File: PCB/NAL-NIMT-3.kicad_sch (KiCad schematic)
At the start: 27 parts

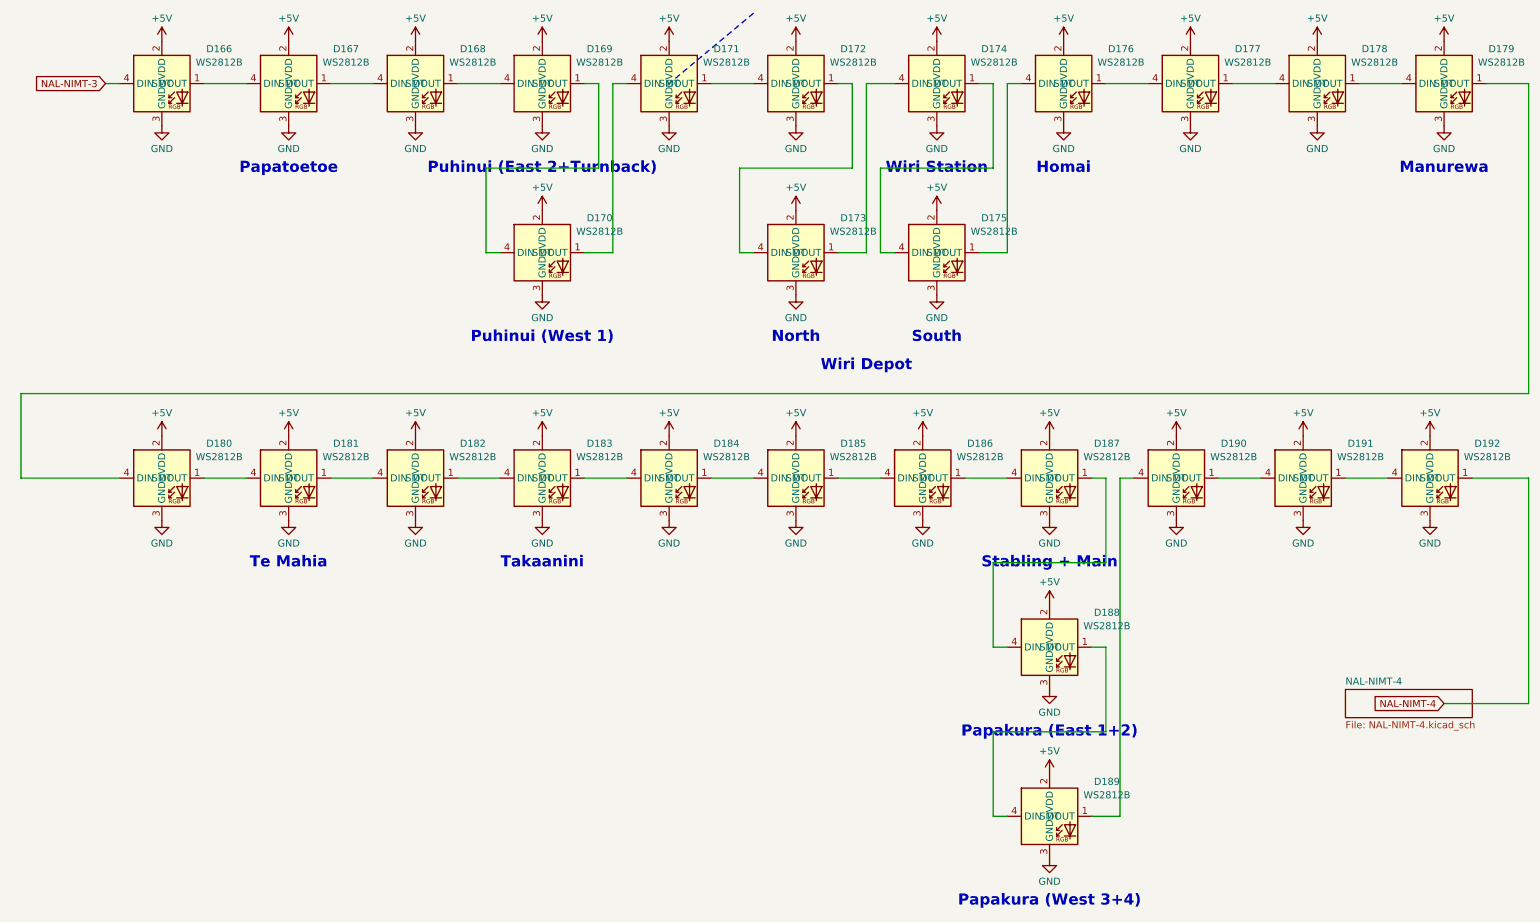
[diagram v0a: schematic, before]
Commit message: V1.1.0 PCB
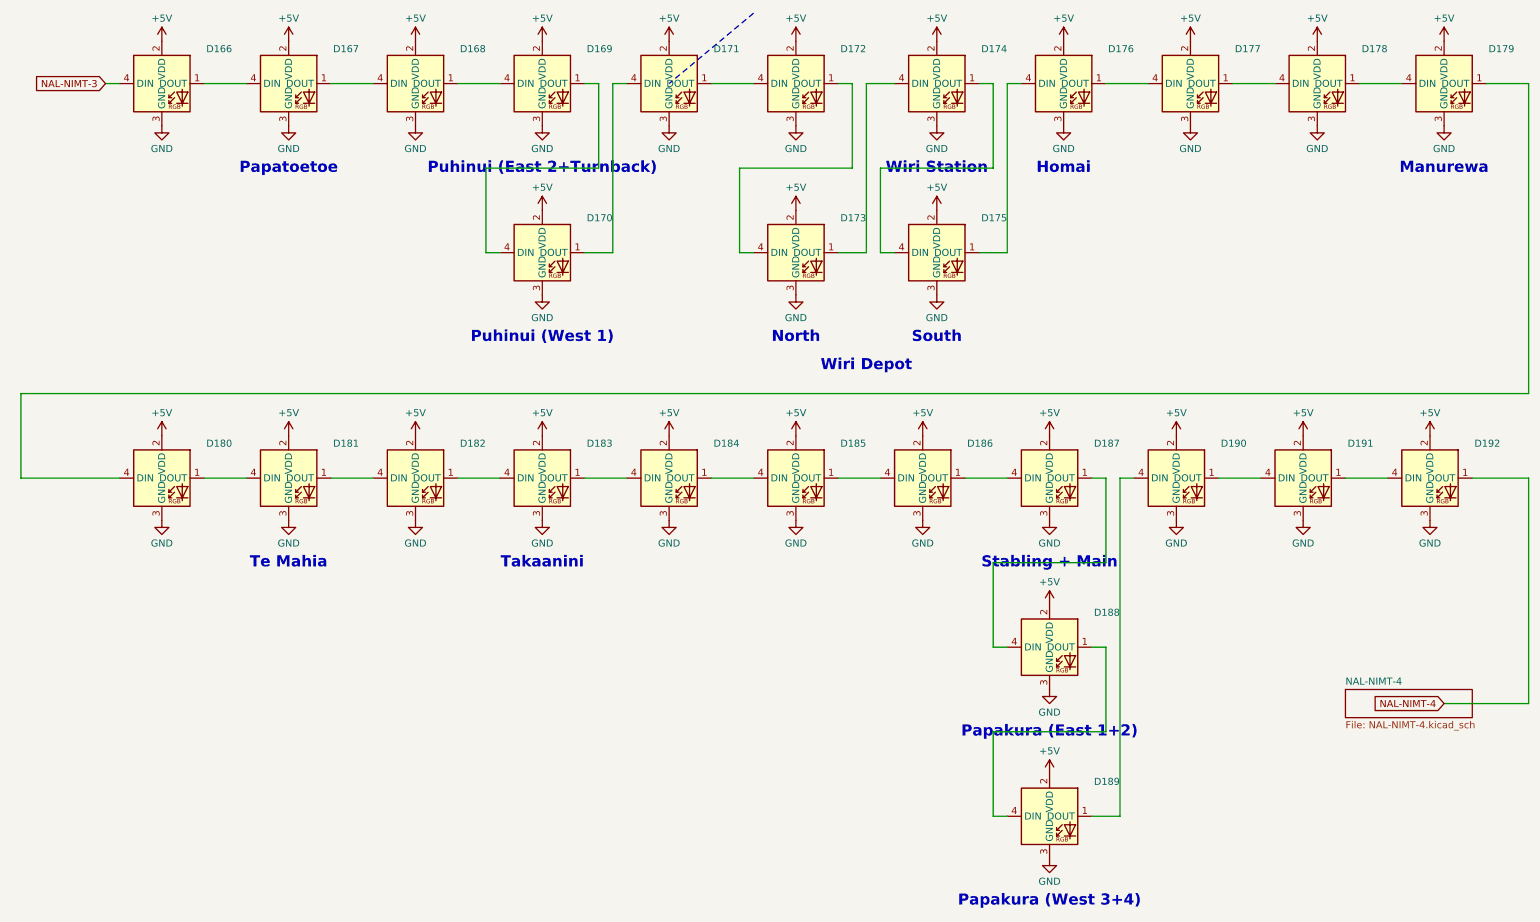
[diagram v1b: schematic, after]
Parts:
- D166, D167, D168, D169, D170, D171, D172, D173, D174, D175, D176, D177, D178, D179, D180, D181, D182, D183, D184, D185, D186, D187, D188, D189, D190, D191, D192: value WS2812B -> XL-1615RGBC-WS2812B-S; LCSC C5349954 -> C41413180; Manufacturer XINGLIGHT -> (none); Part XL-1615RGBC-WS2812B -> (none); Process SMT -> (none)

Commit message: Update to meet OSHWA Certification
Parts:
- D166, D167, D168, D169, D170, D171, D172, D173, D174, D175, D176, D177, D178, D179, D180, D181, D182, D183, D184, D185, D186, D187, D188, D189, D190, D191, D192: Manufacturer (none) -> XINGLIGHT; Part (none) -> XL-1615RGBC-WS2812B-S
